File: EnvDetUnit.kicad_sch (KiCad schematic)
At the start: 19 parts, among them CN1 CON_GROVE, CN2 CON_GROVE, J1 Conn_01x03, J2 Conn_01x03, J3 Conn_01x02, U1 S89431

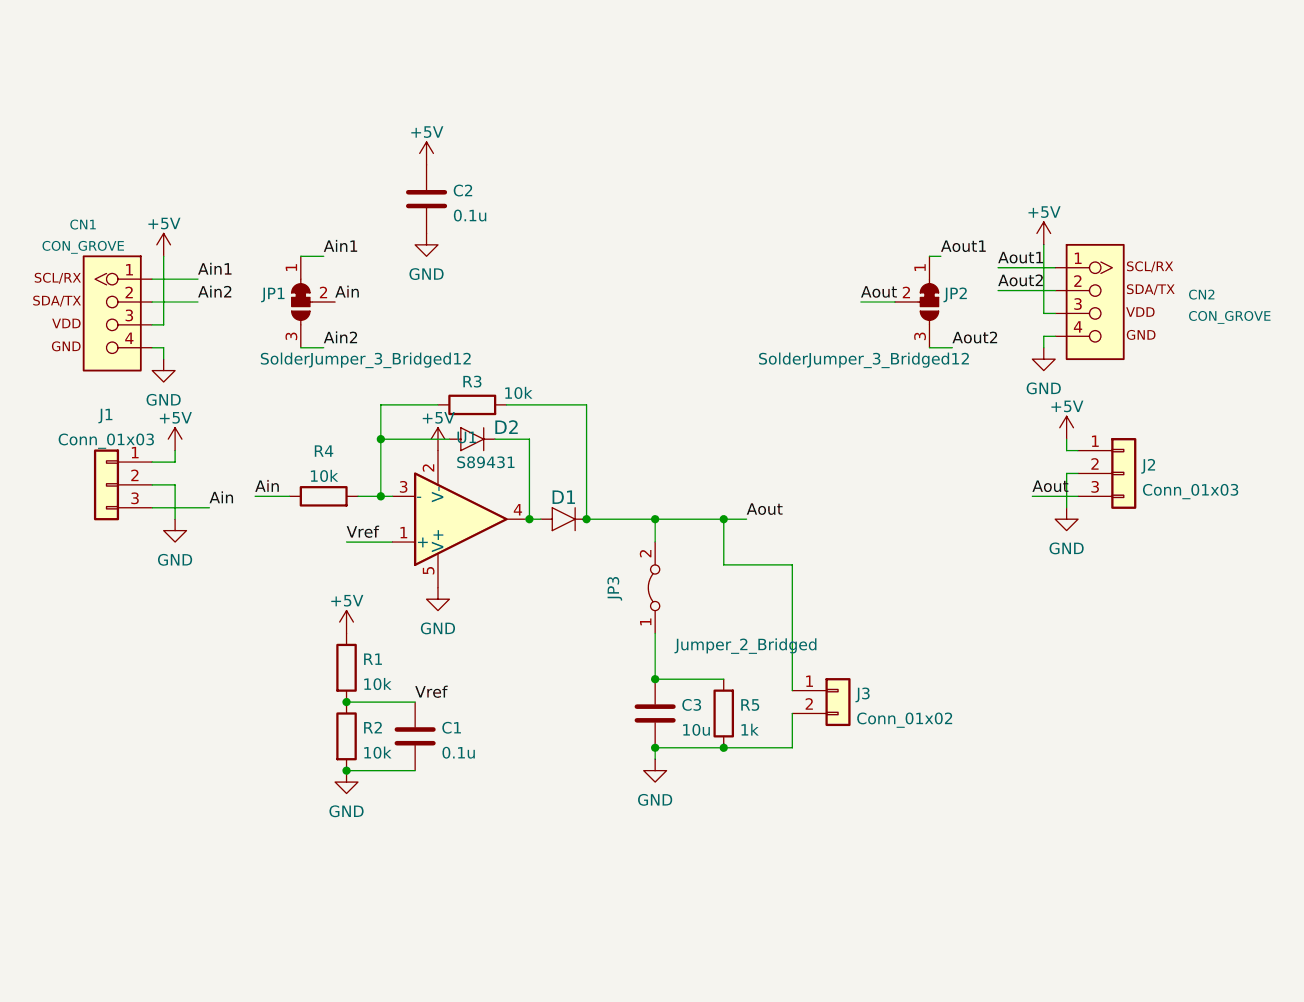
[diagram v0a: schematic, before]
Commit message: update PCB data
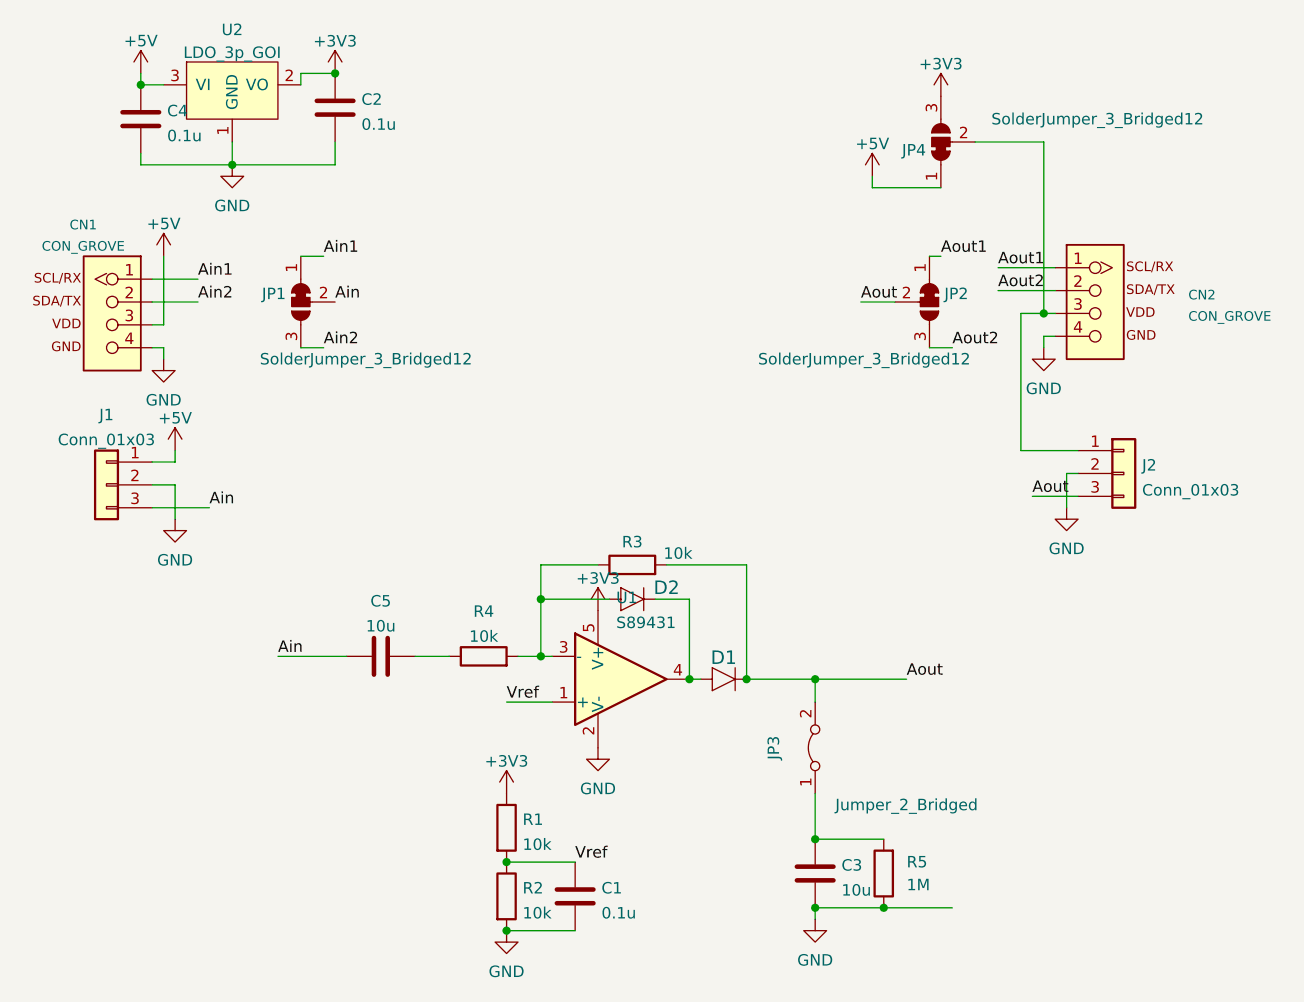
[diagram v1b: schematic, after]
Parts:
- removed J3: Conn_01x02, Connector_PinSocket_2.54mm:PinSocket_1x02_P2.54mm_Vertical, symbol Connector_Generic:Conn_01x02
- added C4: 0.1u, Capacitor_SMD:C_0603_1608Metric, symbol Device:C
- added C5: 10u, Capacitor_SMD:C_0603_1608Metric, symbol Device:C
- added JP4: SolderJumper_3_Bridged12, Jumper:SolderJumper-3_P1.3mm_Bridged2Bar12_Pad1.0x1.5mm_NumberLabels, symbol Jumper:SolderJumper_3_Bridged12
- added U2: LDO_3p_GOI, Package_TO_SOT_SMD:SOT-23, symbol akita:LDO_3p_GOI
- R5: value 1k -> 1M
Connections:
- net +5V: now also C4.1, JP4.1 (A), U2.3 (VI); no longer C2.1, CN2.3, J2.1 (Pin_1), R1.1, U1.2 (V-)
- net Ain: now also C5.1; no longer R4.1
- net GND: now also U1.2 (V-), C4.2, U2.1 (GND); no longer U1.5 (V+)
- new net: CN2.3, J2.1 (Pin_1), JP4.2 (C)
- new net: C5.2, R4.1
- new net +3V3: C2.1, JP4.3 (B), R1.1, U1.5 (V+), U2.2 (VO)
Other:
- moved on the sheet: C1, C2, C3, D1, D2, JP3, R1, R2, R3, R4, R5, U1
